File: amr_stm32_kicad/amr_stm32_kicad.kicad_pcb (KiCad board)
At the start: 4 copper layers, 85 x 56 mm, 96 parts, among them J1 Header 2x20, J10 VCC, J2 Motor_Left, J3 Motor_right, J4 ST_Link, J5 USB_FS_Interface, J6 USB_UART, J7 +12V_BAT, J8 USB_A_Pi, J9 UART, Q1 FDN304P, SW1 SW_Reset, SW2 SW_BOOT, U2 SGM2205-3.3, U3 BMI323, U4 TB6612FNG, U5 STM32F405RGTx, U6 LM358, U7 CH340E, U9 TPS56528DDA, Y2 8MHz

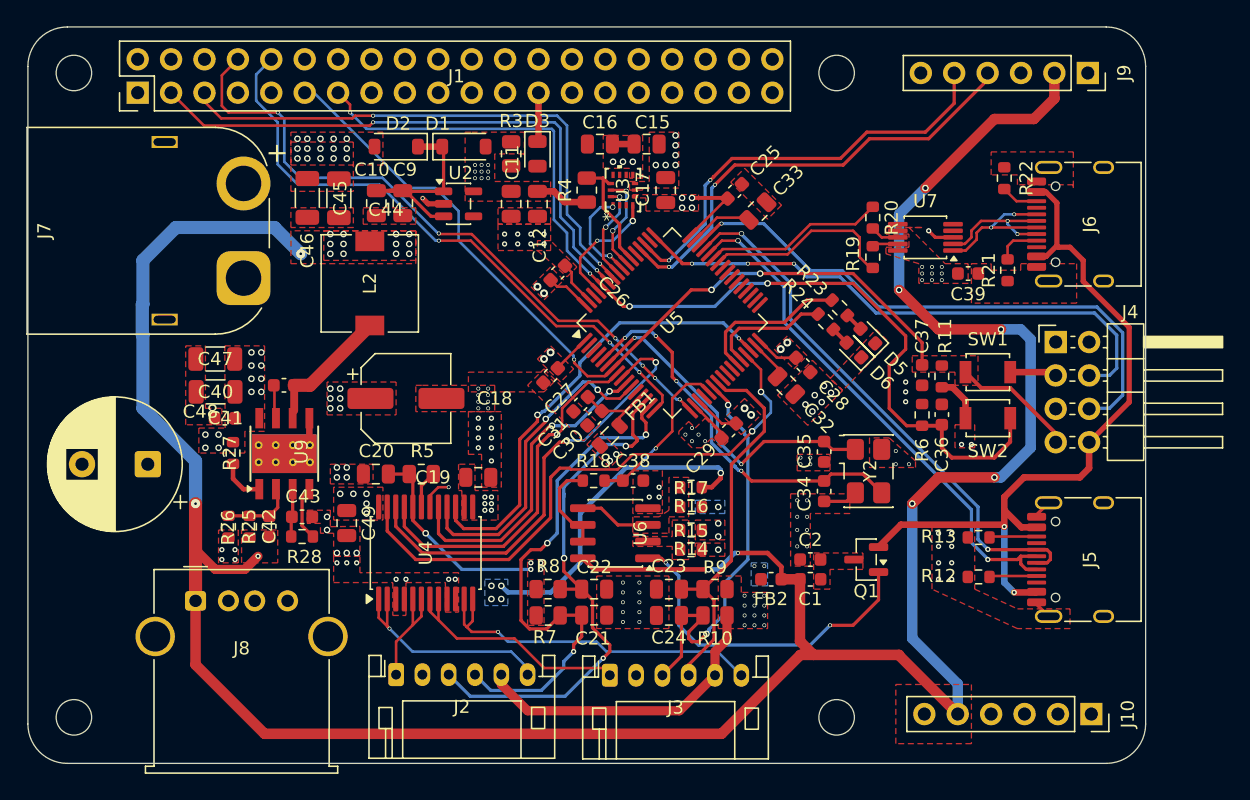
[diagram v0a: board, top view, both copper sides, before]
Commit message: update14
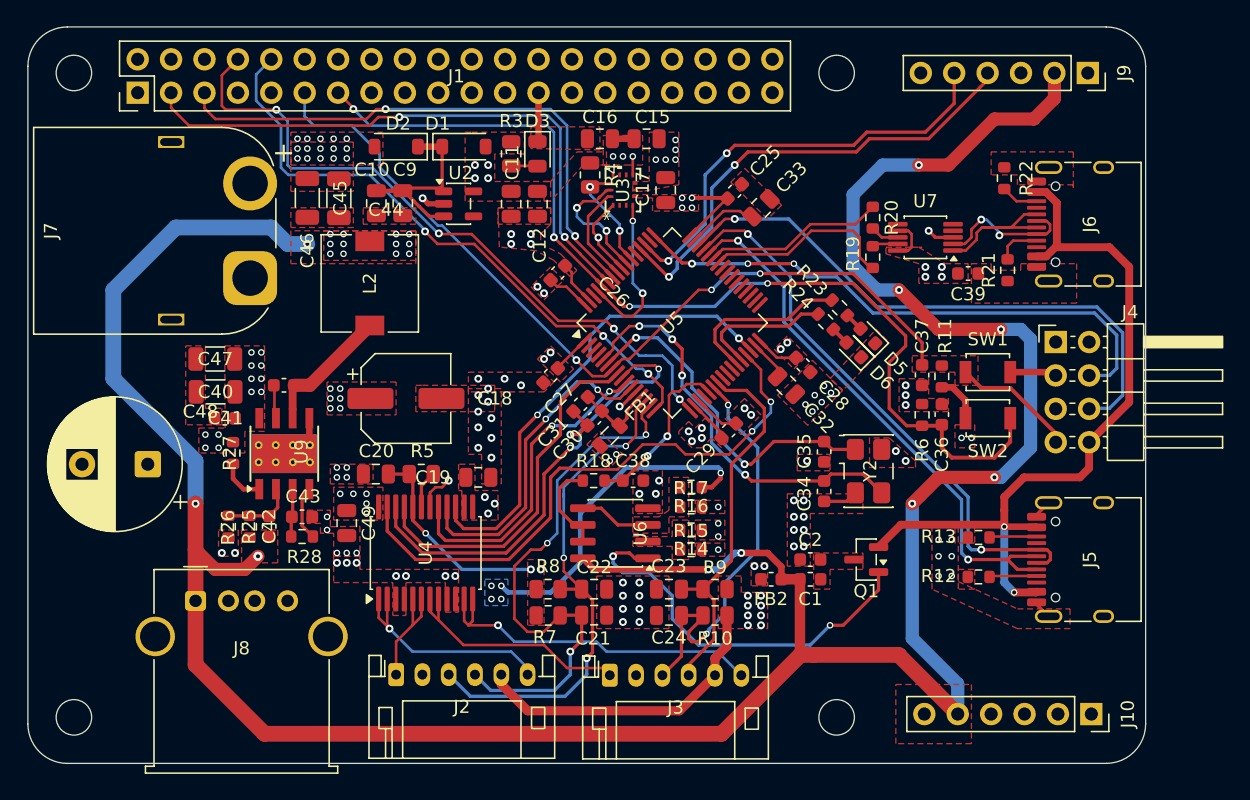
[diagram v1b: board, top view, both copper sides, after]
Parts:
- U3: footprint BMI323:BMI323_BOS -> BMI323:BMI323_BOS-L
- moved R4 1.18 mm to (162.0, 61.2), turned to -90 degrees
- moved J7 0.50 mm to (136.2, 69.1)
- moved C15 0.41 mm to (166.3, 58.5)
- moved C16 0.41 mm to (162.8, 58.5)
- moved C33 0.35 mm to (175.0, 63.8)
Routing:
- net +5V: track 212.8 -> 221.2 mm
- net GND: track 28.0 -> 33.4 mm, vias 108 -> 89
- net Net-(Q1-G): track 26.0 -> 30.3 mm
- net /IMU_INT: track 9.45 -> 12.5 mm
- net /IMU_SCK: track 7.52 -> 9.62 mm
- net Net-(D3-A): track 0.00 -> 2.01 mm
- net /ENC_1A: track 41.0 -> 39.3 mm
- net /USART2_RX: track 51.2 -> 52.7 mm, vias 6 -> 4
- net /+3.3VA: track 8.33 -> 6.83 mm
- net /USB_DM: track 40.5 -> 42.0 mm
- net /ENC_1B: track 40.8 -> 42.2 mm
- net Net-(U5-PH0): track 29.9 -> 31.2 mm
- net /LED_RUN: track 11.9 -> 13.1 mm
- net VBUS: track 58.0 -> 59.2 mm
- net /LED_ERR: track 9.36 -> 10.6 mm
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- removed copper zone on B.Cu, net GND
